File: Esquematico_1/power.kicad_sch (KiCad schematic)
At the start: 22 parts, among them IC1 AP2112K-3.3TRG1, U6 TPS54302DDCR

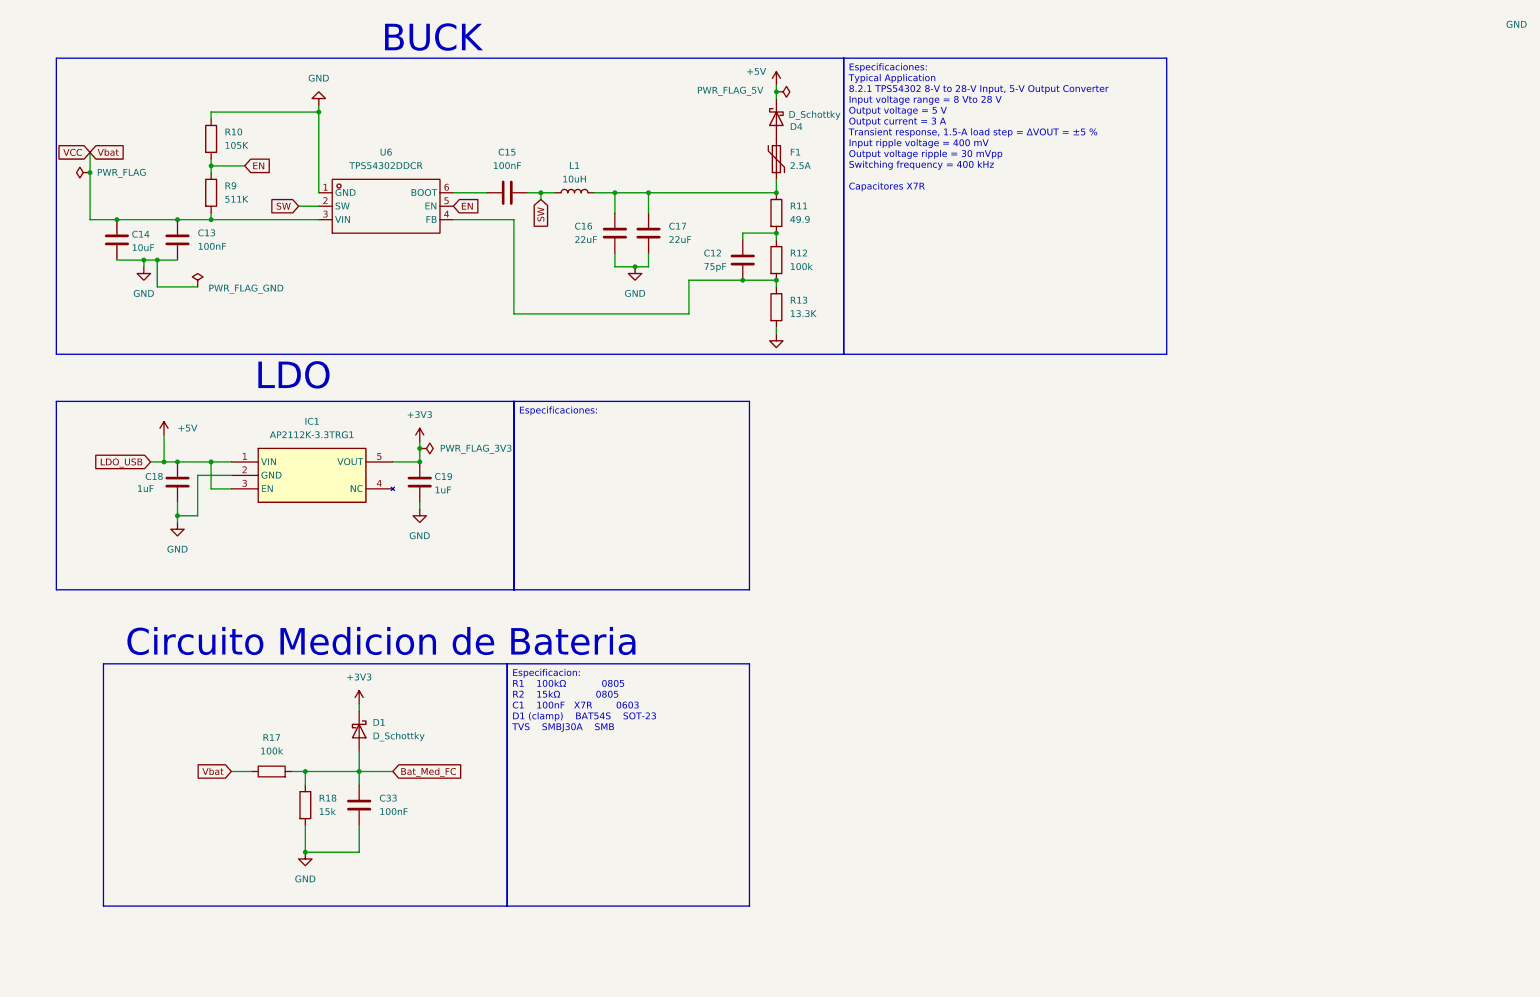
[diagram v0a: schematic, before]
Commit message: Add: Dos bucks :(
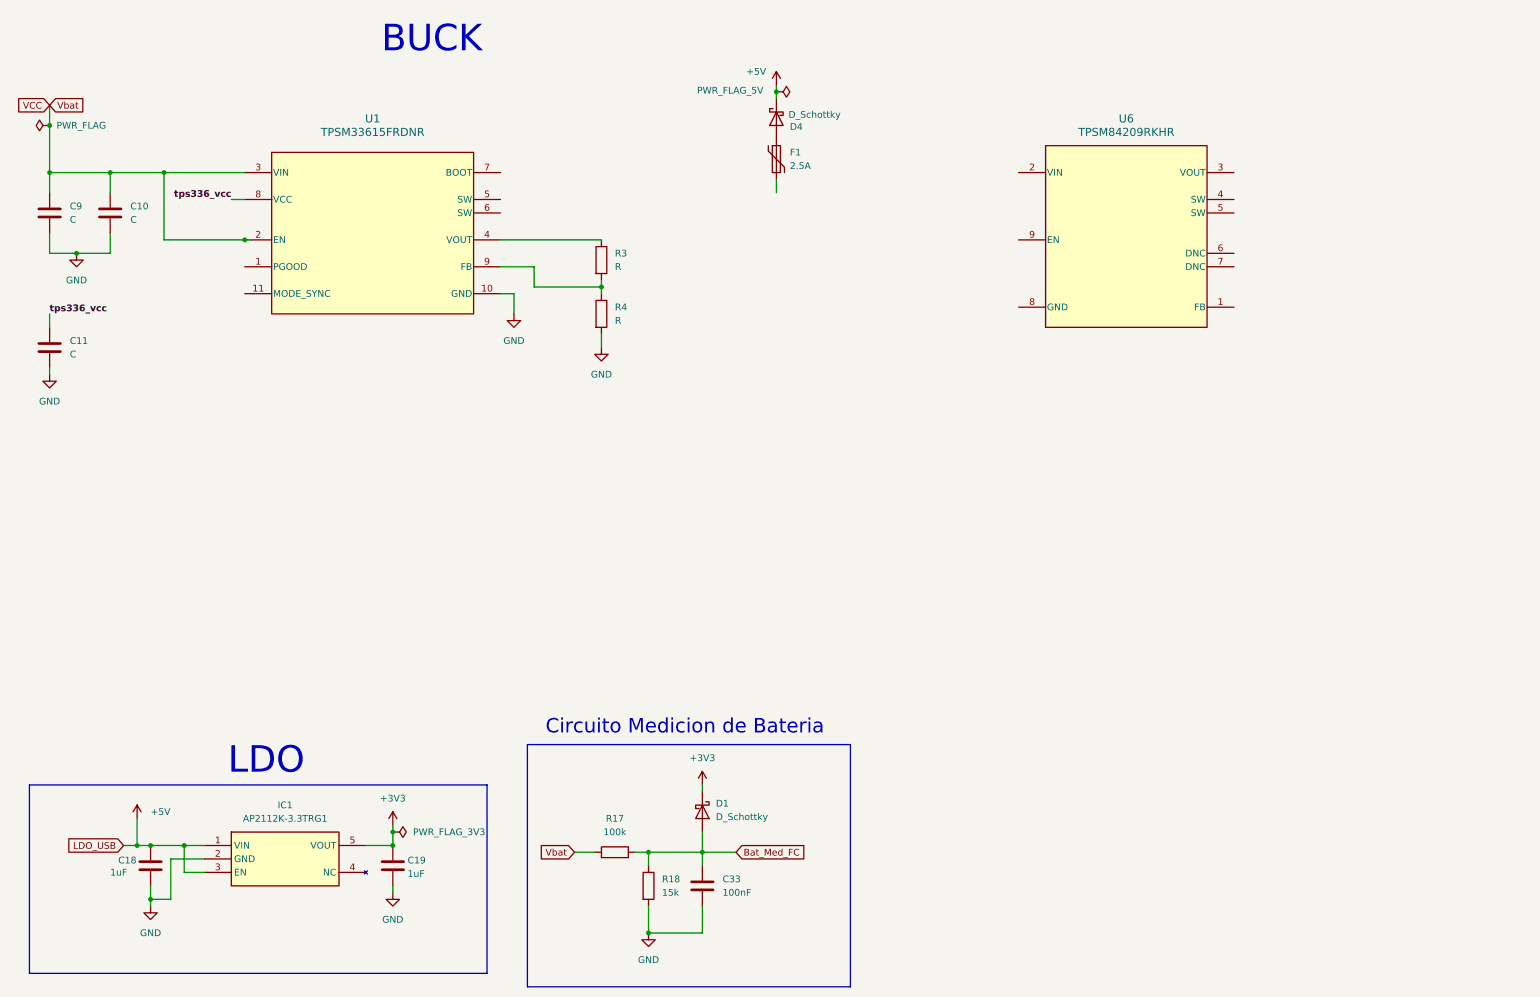
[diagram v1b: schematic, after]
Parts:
- removed C12: 75pF, Capacitor_SMD:C_0805_2012Metric_Pad1.18x1.45mm_HandSolder, symbol Device:C
- removed C13, C15: 100nF, Capacitor_SMD:C_0805_2012Metric_Pad1.18x1.45mm_HandSolder, symbol Device:C
- removed C14: 10uF, Capacitor_SMD:C_0805_2012Metric_Pad1.18x1.45mm_HandSolder, symbol Device:C
- removed C16, C17: 22uF, Capacitor_SMD:C_0805_2012Metric_Pad1.18x1.45mm_HandSolder, symbol Device:C
- removed L1: 10uH, Inductor_SMD:L_KOHERelec_MDA7030, symbol Device:L
- removed R10: 105K, Resistor_SMD:R_0805_2012Metric_Pad1.20x1.40mm_HandSolder, symbol Device:R
- removed R11: 49.9, Resistor_SMD:R_0805_2012Metric_Pad1.20x1.40mm_HandSolder, symbol Device:R
- removed R12: 100k, Resistor_SMD:R_0805_2012Metric_Pad1.20x1.40mm_HandSolder, symbol Device:R
- removed R13: 13.3K, Resistor_SMD:R_0805_2012Metric_Pad1.20x1.40mm_HandSolder, symbol Device:R
- removed R9: 511K, Resistor_SMD:R_0805_2012Metric_Pad1.20x1.40mm_HandSolder, symbol Device:R
- removed U6: TPS54302DDCR, TPS54302DDCR:SOT-23-6_L2.9-W1.6-P0.95-LS2.8-BL, symbol TPS54302DDCR:TPS54302DDCR_C311983
- added C10, C11, C9: C, symbol Device:C
- added R3, R4: R, symbol Device:R
- added U1: TPSM33615FRDNR, RDN0011A-MFG, symbol TPSM33615FRDNR:TPSM33615FRDNR
- added U6: TPSM84209RKHR, RKH0009A, symbol TPSM84209RKHR:TPSM84209RKHR
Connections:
- net GND: now also C10.2, C11.2, C9.2, R4.2, U1.10 (GND)
- net VCC: now also C10.1, C9.1, U1.2 (EN), U1.3 (VIN)
- new net: R3.2, R4.1, U1.9 (FB)
- new net: R3.1, U1.4 (VOUT)
- new net tps336_vcc: C11.1, U1.8 (VCC)
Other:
- moved on the sheet: C18, C19, C33, D1, IC1, R17, R18
